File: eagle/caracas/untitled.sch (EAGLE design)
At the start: 18 parts, among them IC1 4001N, Q1 IRLZ44Z, X1 22-23-2021, X2 22-23-2021, X3 22-23-2041, X4 22-23-2041, X5 22-23-2021, X6 22-23-2021

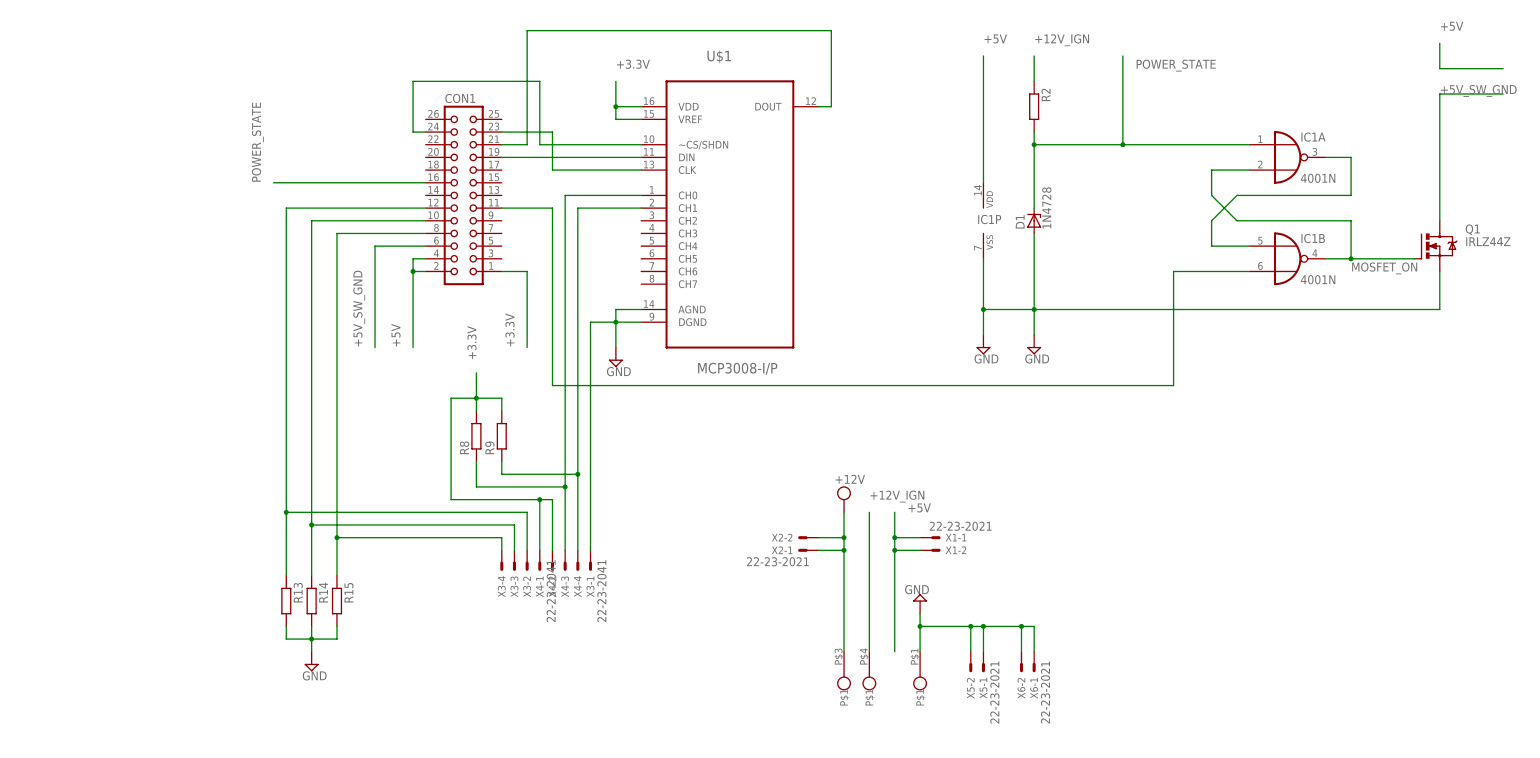
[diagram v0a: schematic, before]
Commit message: Update schematics again.
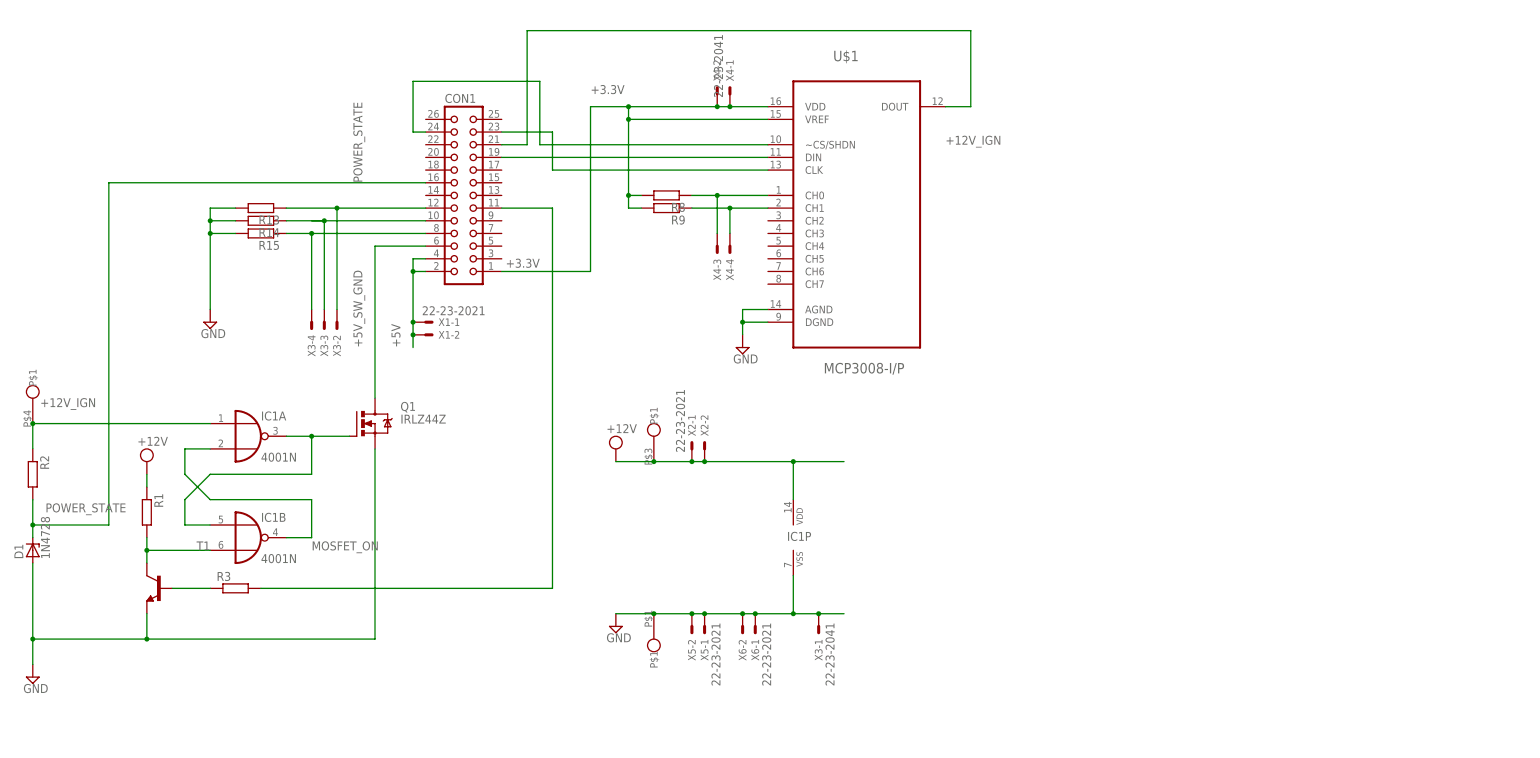
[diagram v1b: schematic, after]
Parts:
- added R1, R3: (no value), rcl:R-EU_0207/10
- added T1: (no value), transistor:MPS2222A-NPN-TO92-CBE
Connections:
- new net N$2: IC1B.I1, R1.2, T1.C
- new net N$9: R3.1, T1.B
- net +12V_IGN: now also IC1A.I0
- net +5V: no longer IC1P.VDD
- net GND: now also T1.E
- net MOSFET_ON: no longer Q1.G
- net N$1: now also Q1.G
- net POWER_STATE: no longer IC1A.I0
- net RPI_RESET: now also R3.2; no longer IC1B.I1
- net VCC: now also IC1P.VDD, R1.1
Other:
- moved on the sheet: D1, IC1A, IC1B, IC1P, Q1, R13, R14, R15, R2, R8, R9, U$1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
